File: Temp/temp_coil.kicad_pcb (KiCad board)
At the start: 2 copper layers, 0 parts

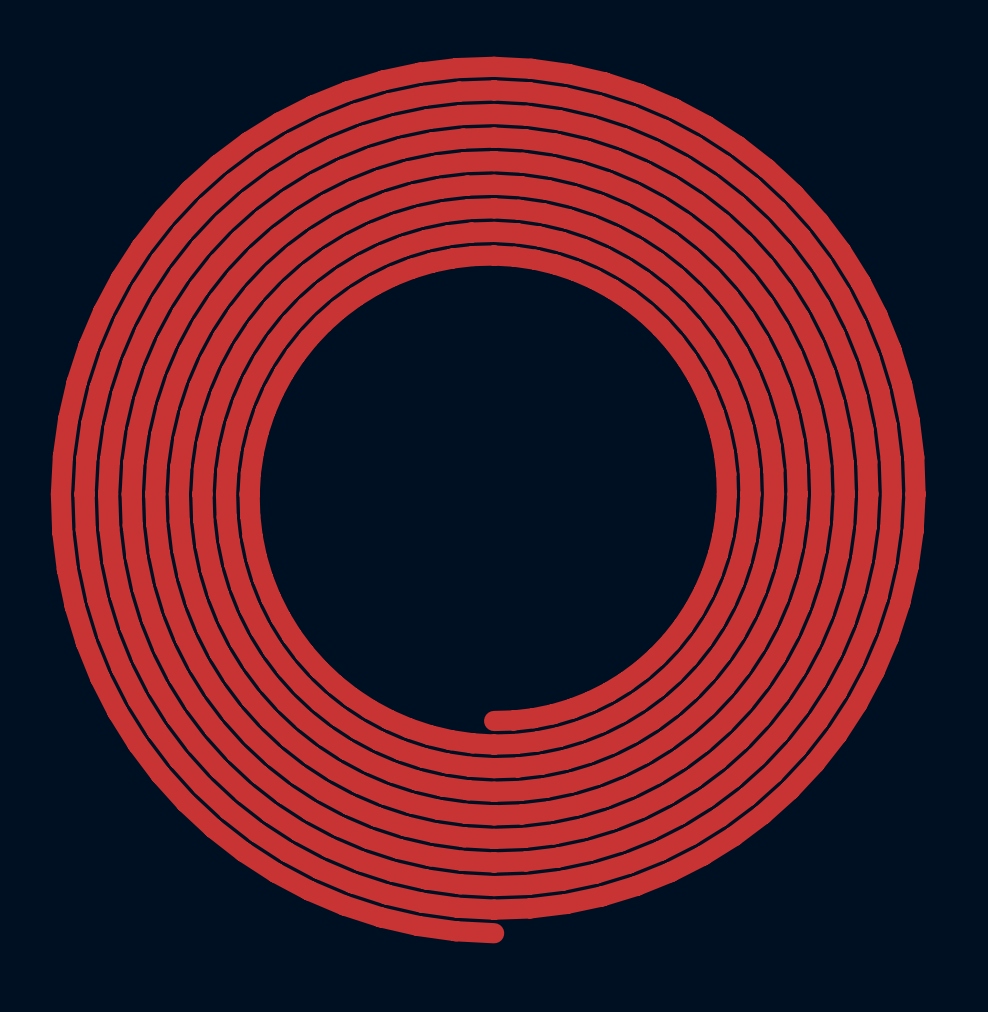
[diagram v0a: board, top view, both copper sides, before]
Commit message: Working pcbnew
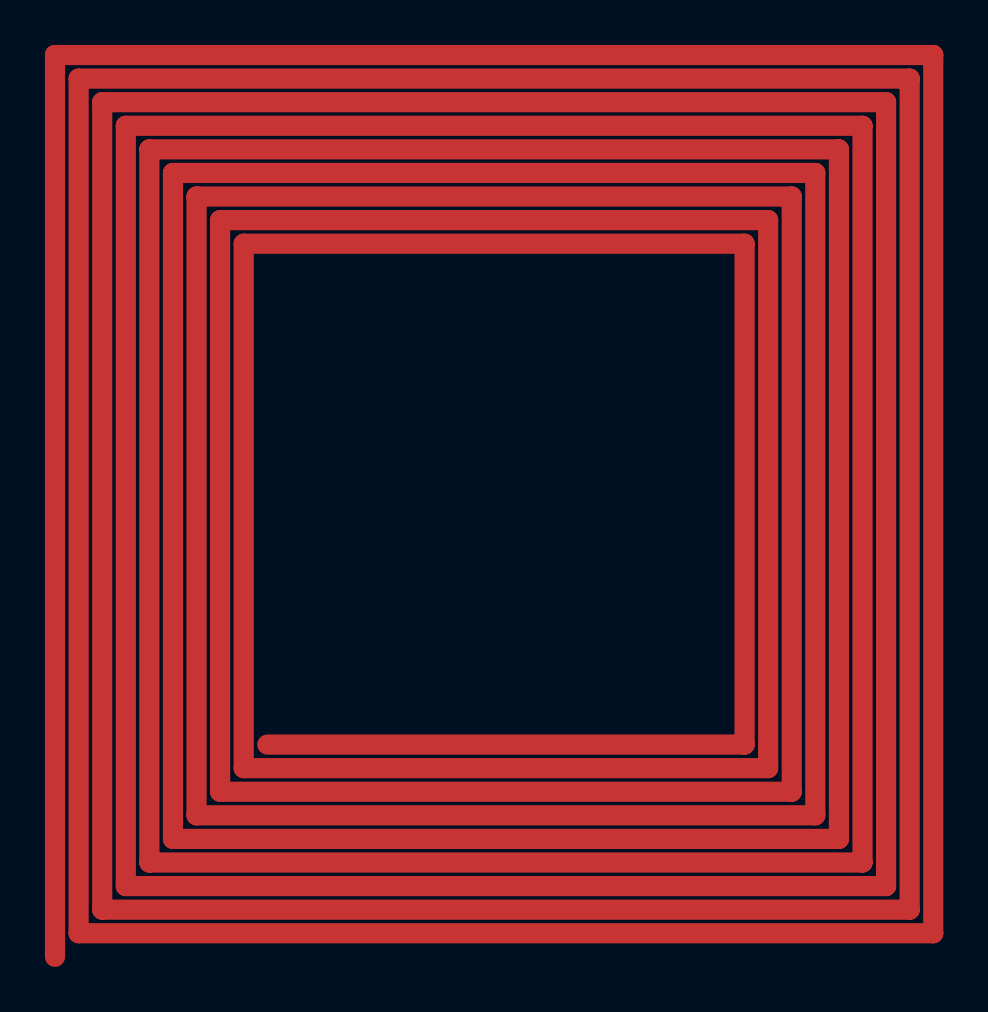
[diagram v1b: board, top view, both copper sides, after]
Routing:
- net (no net): track 838.1 -> 1105.2 mm
